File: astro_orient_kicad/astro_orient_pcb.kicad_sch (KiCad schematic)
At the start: 33 parts, among them J1 BME260, J2 SWD_Tag_Connect, J3 USB-C_Receptacle, J4 test_points, SW1 SW_SPST, SW2 SW_Reset, SW3 SW_Boot, U1 STM32F072CBTx, U2 AP2112K-3.3, Y1 osc_crystal

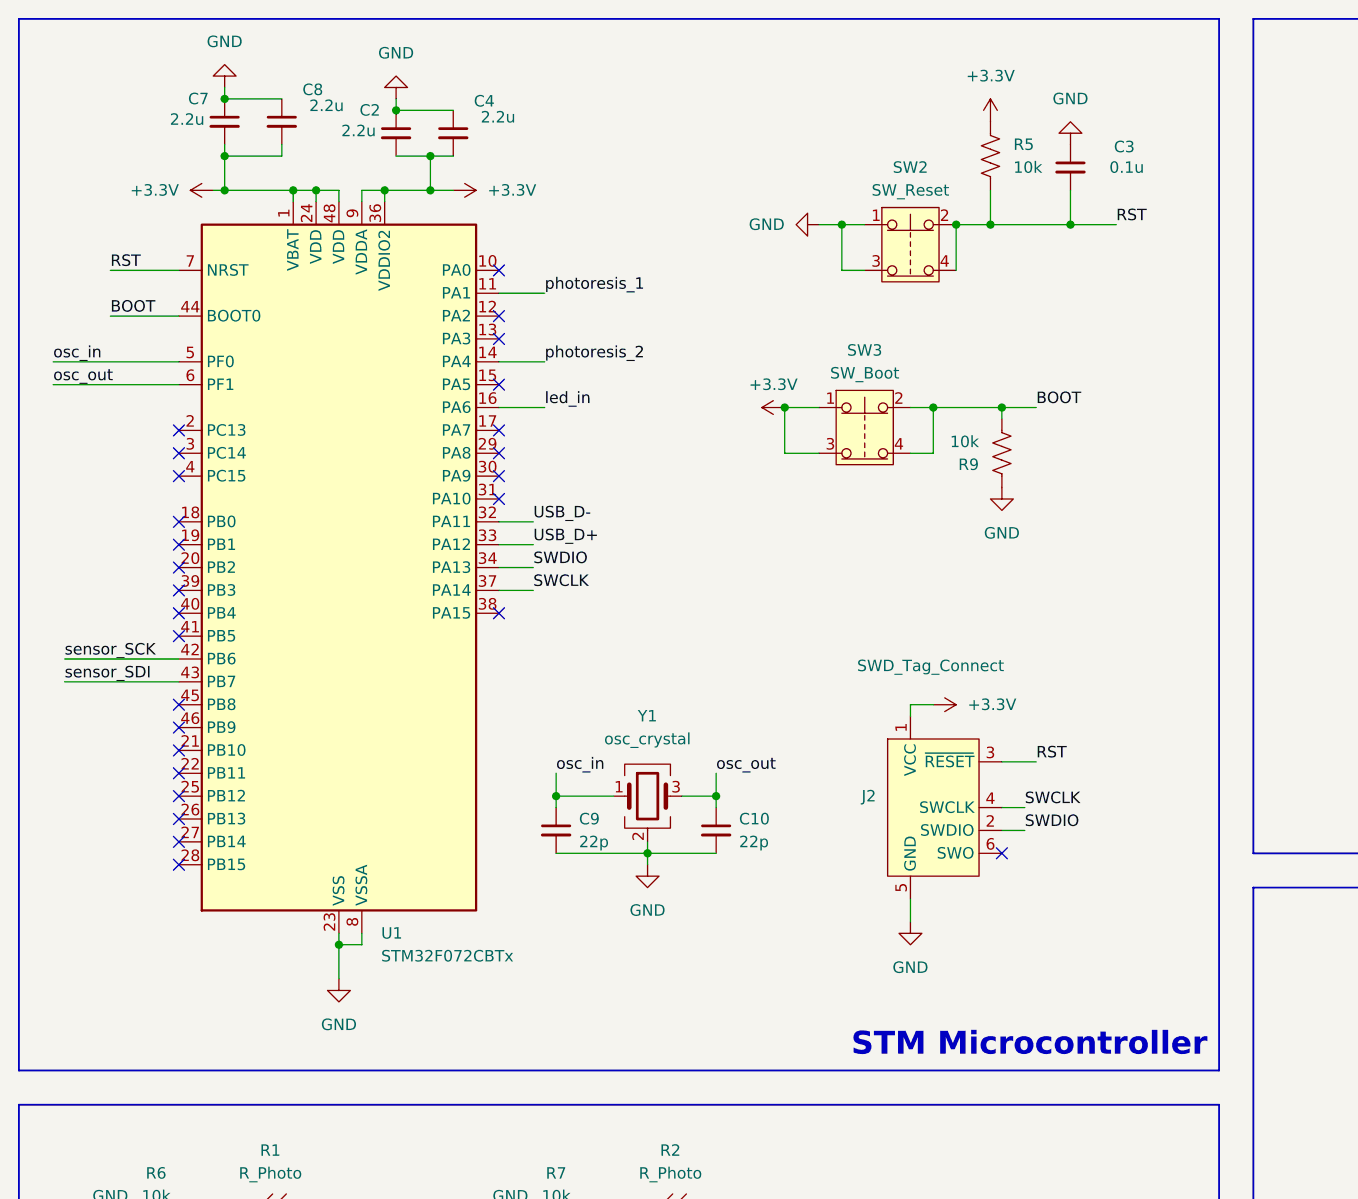
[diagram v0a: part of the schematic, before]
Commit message: Updated PCB schematic
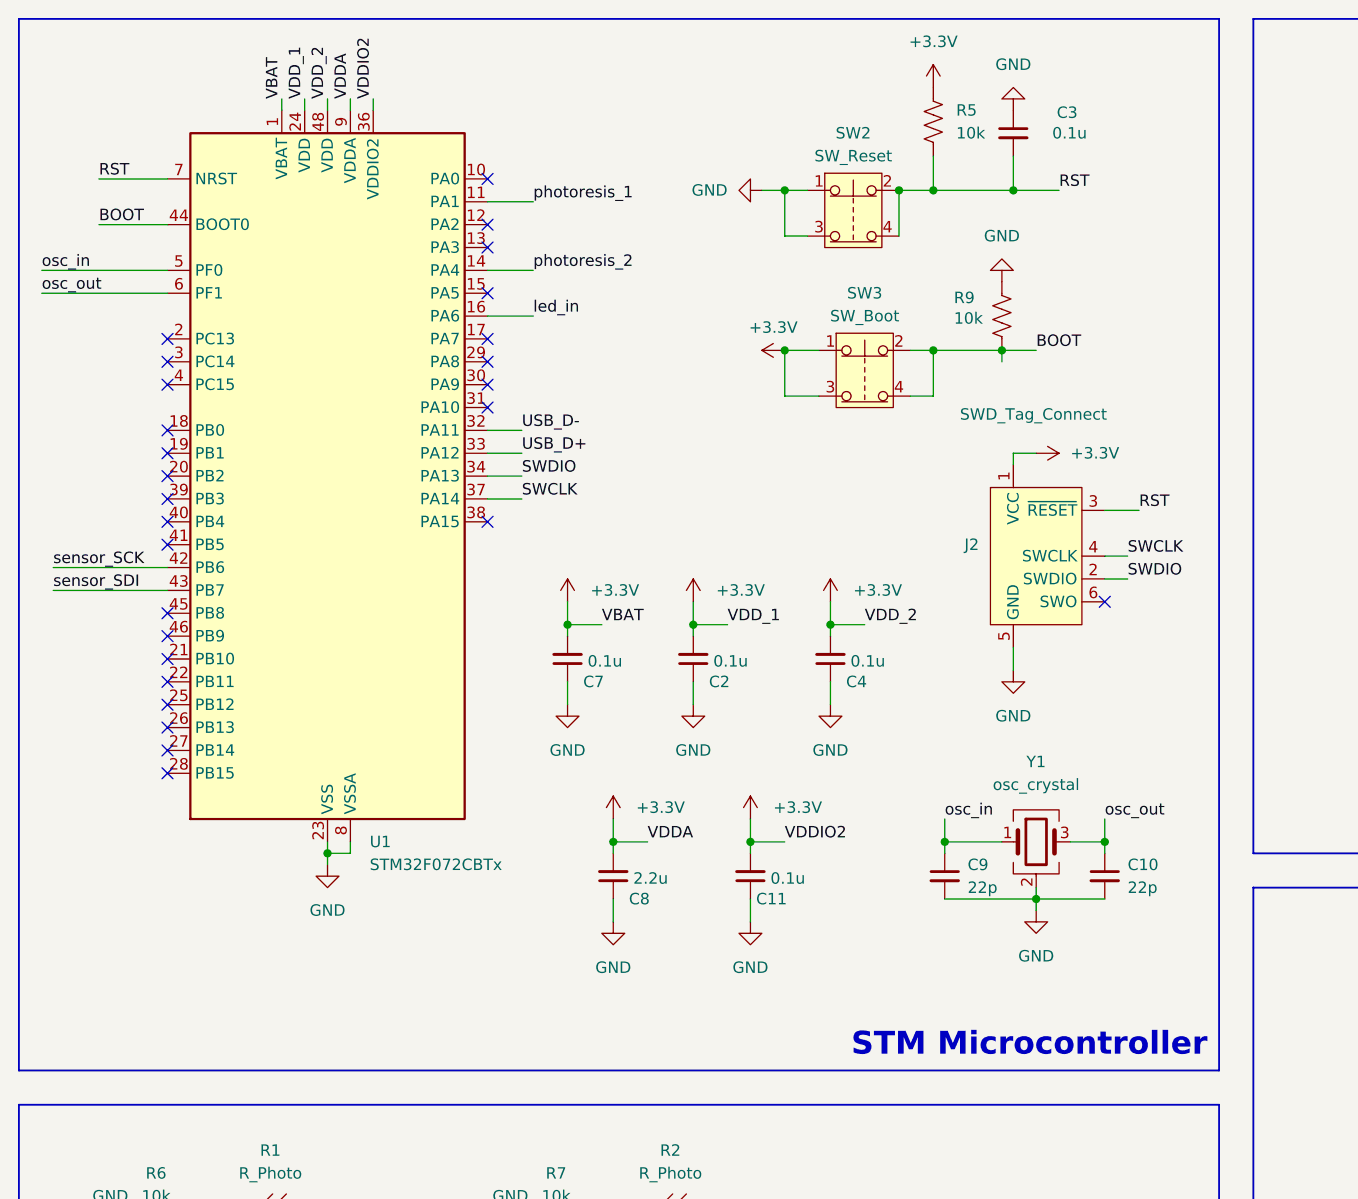
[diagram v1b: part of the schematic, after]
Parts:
- added C11: 0.1u, symbol Device:C_Small
- C2, C4, C7: value 2.2u -> 0.1u
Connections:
- net +3.3V: now also C11.2
- net GND: now also C11.1
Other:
- moved on the sheet: C10, C3, C7, C9, J2, R5, R9, SW2, SW3, U1, Y1
